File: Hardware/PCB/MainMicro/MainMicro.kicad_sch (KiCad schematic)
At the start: 15 parts

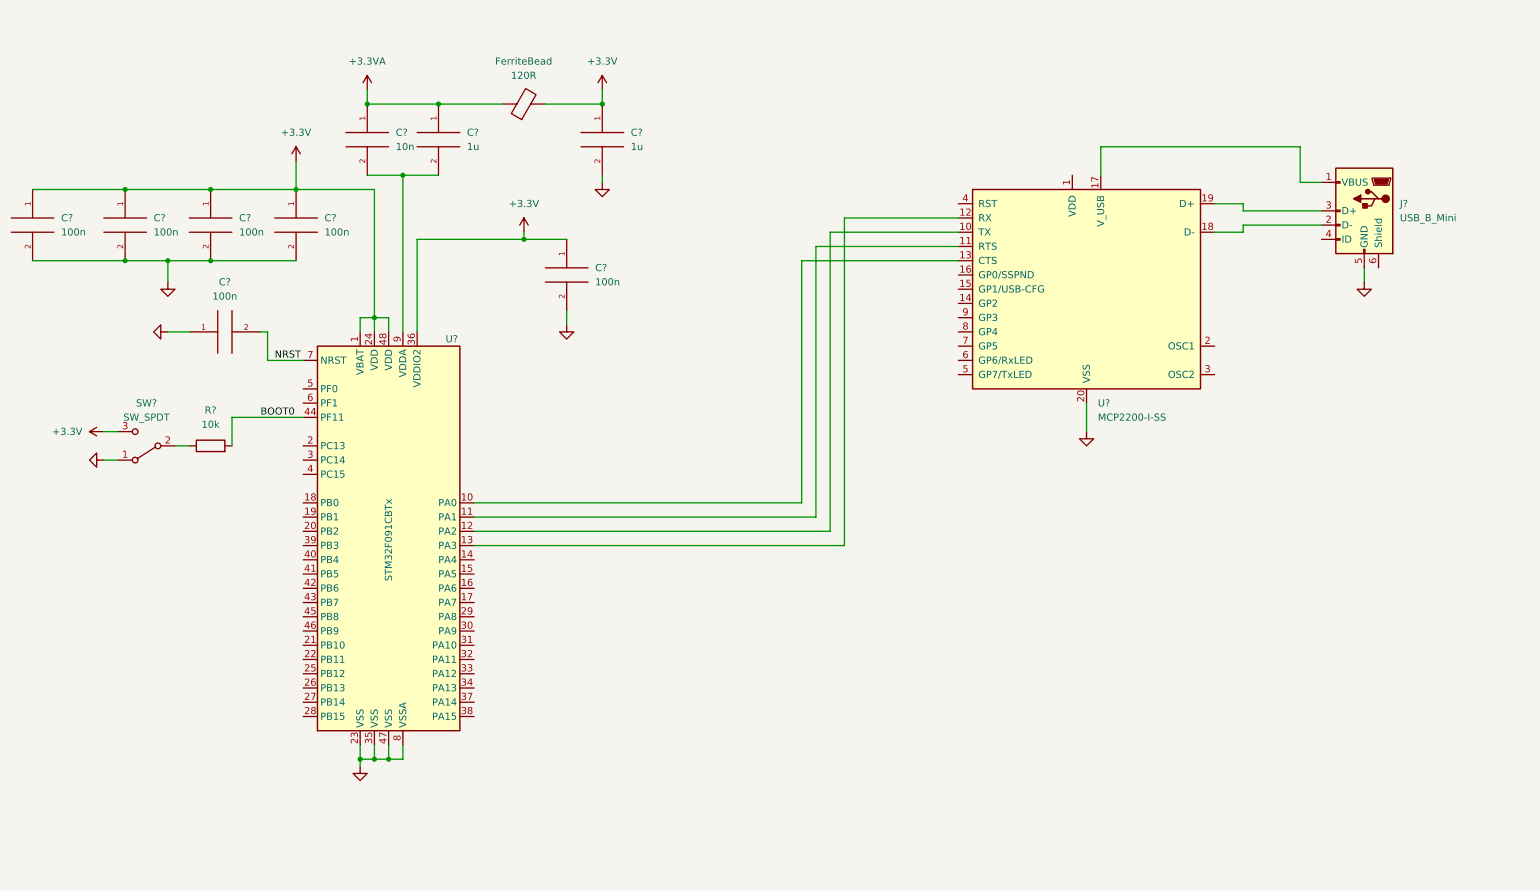
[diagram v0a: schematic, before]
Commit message: More PCB stuff
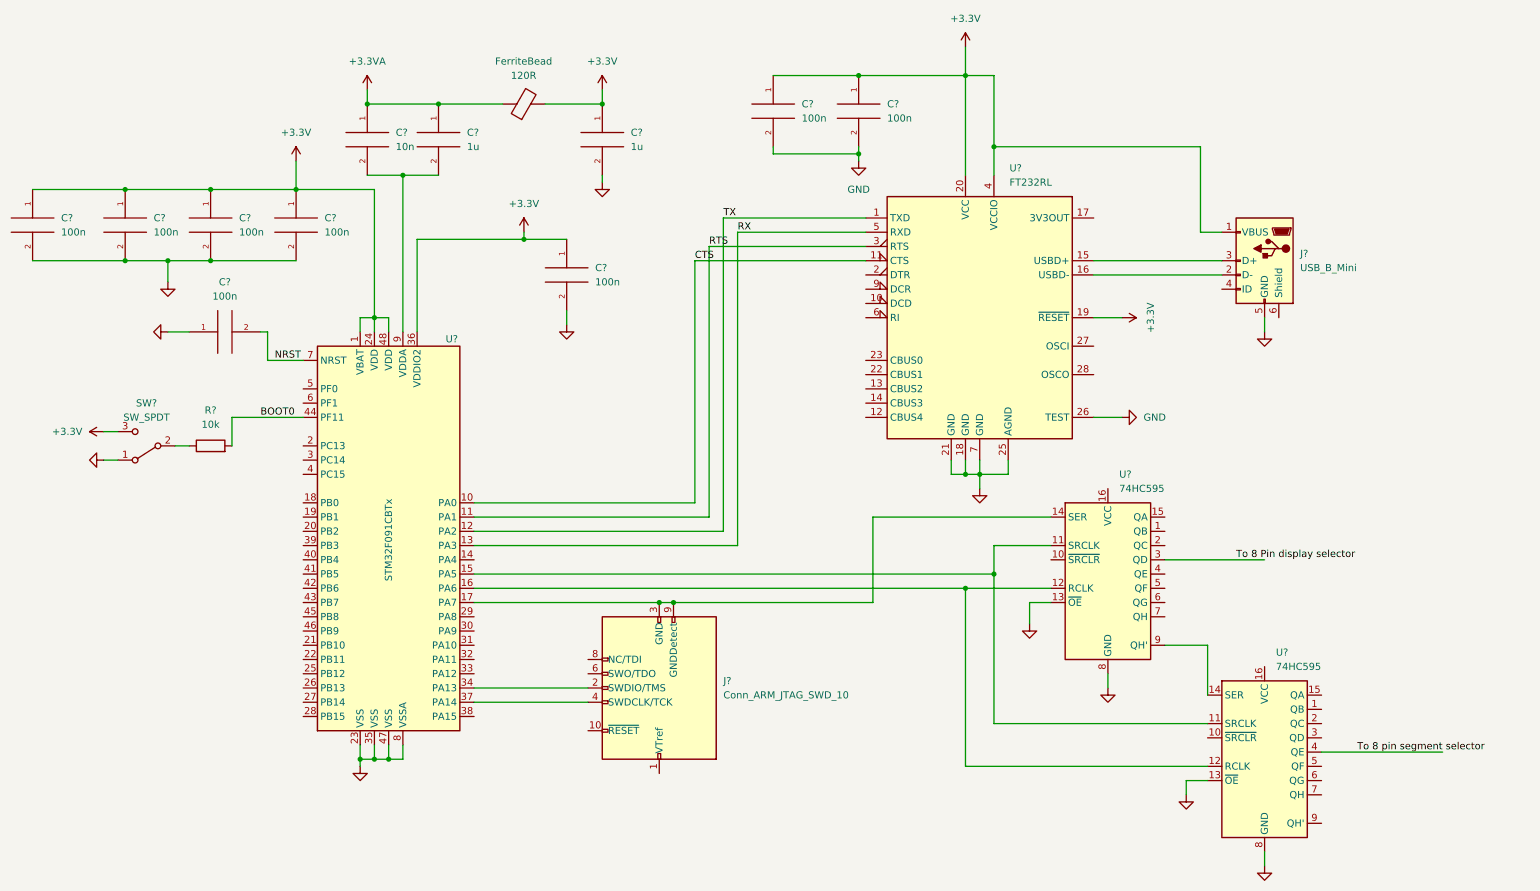
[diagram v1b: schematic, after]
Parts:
- removed U?: MCP2200-I-SS, Package_SO:SSOP-20_5.3x7.2mm_P0.65mm, symbol Interface_USB:MCP2200-I-SS
- added C? (x2): 100n, symbol pspice:C
- added J?: Conn_ARM_JTAG_SWD_10, symbol Connector:Conn_ARM_JTAG_SWD_10
- added U? (x2): 74HC595, symbol 74xx:74HC595
- added U?: FT232RL, Package_SO:SSOP-28_5.3x10.2mm_P0.65mm, symbol Interface_USB:FT232RL
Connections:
- net +3V3: now also J?.1 (VBUS), C?.1, C?.1, U?.19 (~{RESET}), U?.20 (VCC), U?.4 (VCCIO)
- net GND: now also C?.2, C?.2, U?.13 (~{OE}), U?.13 (~{OE}), U?.18 (GND), U?.21 (GND), U?.25 (AGND), U?.26 (TEST), U?.7 (GND), U?.8 (GND), U?.8 (GND)
- net CTS: now reaches U?.10 (PA0)
- net CTS: now also U?.11 (CTS)
- net RTS: now reaches U?.11 (PA1)
- net RTS: now also U?.3 (RTS)
- net TX: now reaches U?.12 (PA2)
- net TX: now also U?.1 (TXD)
- net RX: now reaches U?.13 (PA3)
- net RX: now also U?.5 (RXD)
- net at U?.15 (PA5): now also U?.11 (SRCLK), U?.11 (SRCLK)
- net at U?.16 (PA6): now also U?.12 (RCLK), U?.12 (RCLK)
- net at U?.17 (PA7): now also J?.3 (GND), J?.5 (GND), J?.9 (GNDDetect), U?.14 (SER)
- net at U?.34 (PA13): now also J?.2 (SWDIO/TMS)
- net at U?.37 (PA14): now also J?.4 (SWDCLK/TCK)
- net at J?.2 (D-): now also U?.16 (USBD-)
- net at J?.3 (D+): now also U?.15 (USBD+)
- new net: U?.14 (SER), U?.9 (QH')
- new net To 8 Pin display selector: U?.3 (QD)
- new net To 8 pin segment selector: U?.4 (QE)
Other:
- moved on the sheet: J?
